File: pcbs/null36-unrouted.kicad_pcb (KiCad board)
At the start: 2 copper layers, 123.2 x 106.1 mm, 40 parts

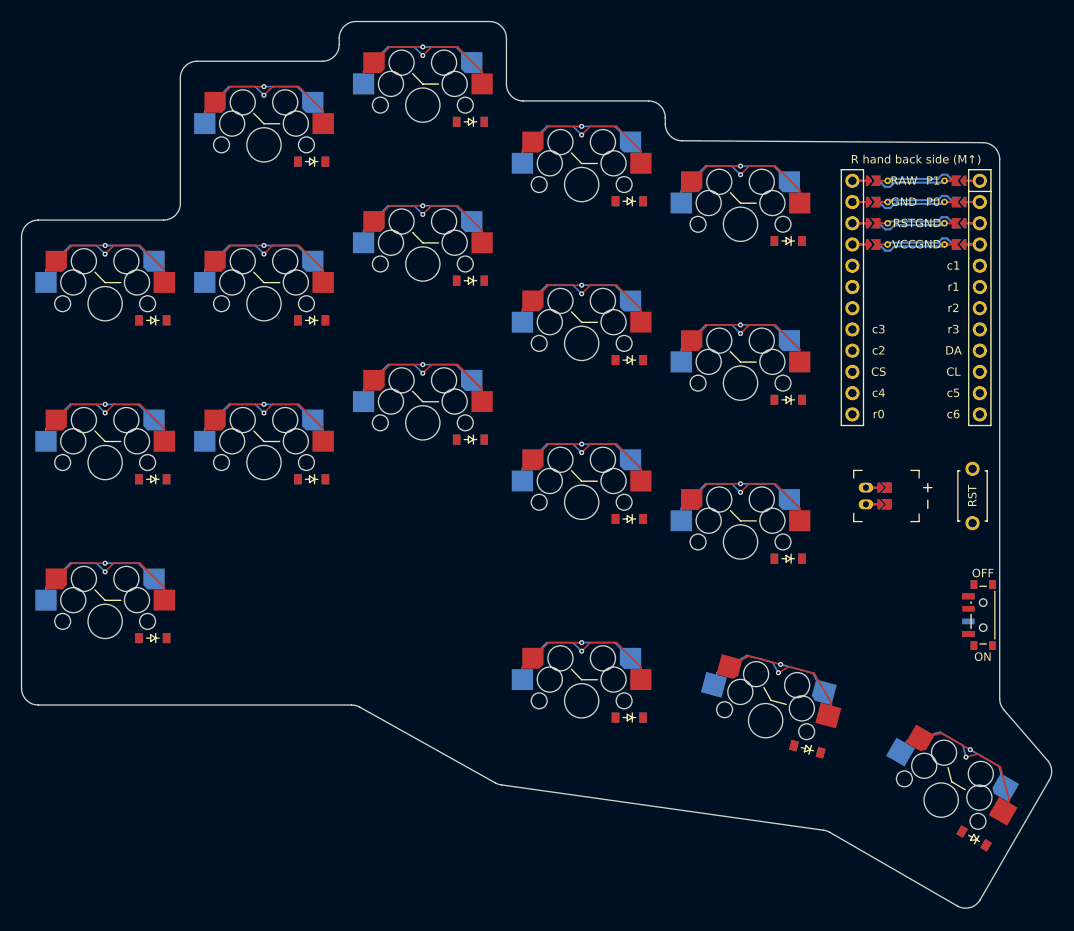
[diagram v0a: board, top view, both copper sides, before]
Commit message: v3 pcb design
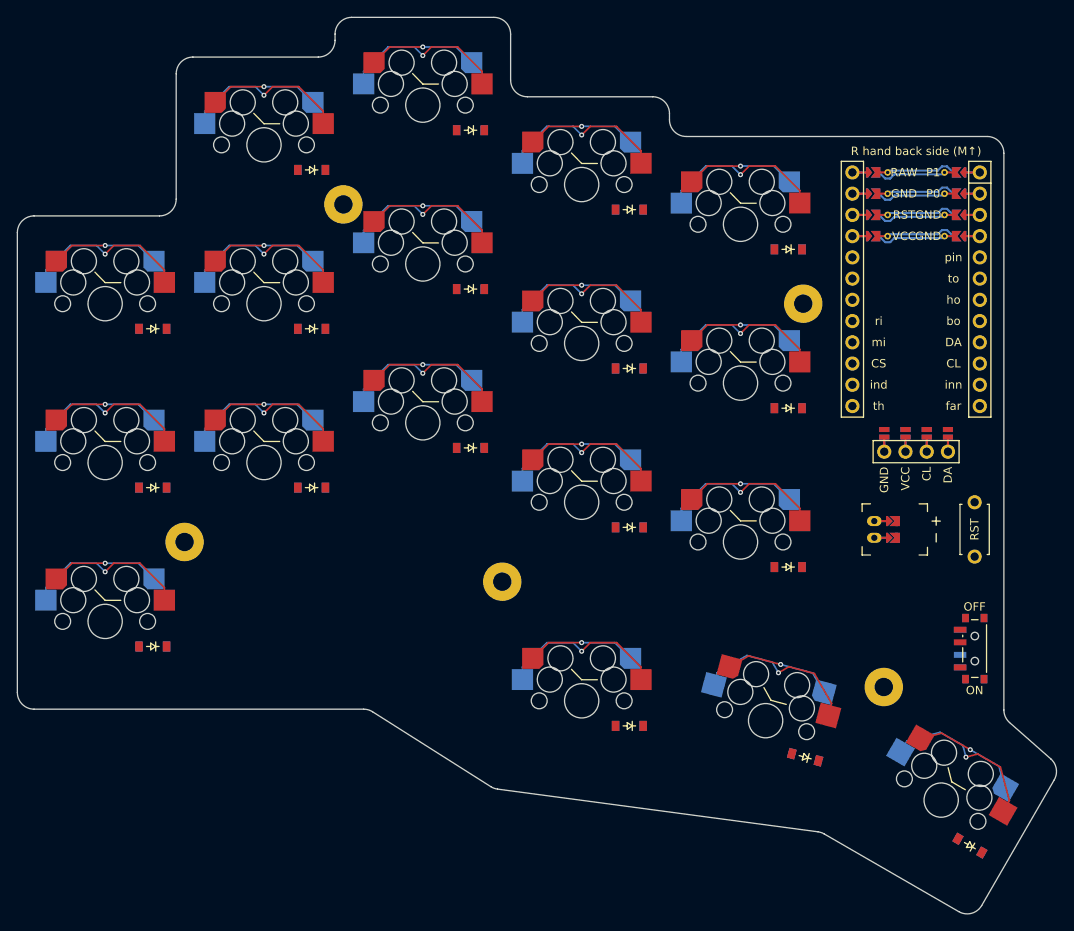
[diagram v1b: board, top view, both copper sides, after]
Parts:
- added DISP1: , ceoloide:display_ssd1306, F.Cu at (247.0, 113.0)
- added MH1: , ceoloide:mounting_hole_npth, F.Cu at (159.5, 140.5)
- added MH2: , ceoloide:mounting_hole_npth, F.Cu at (178.5, 100.1)
- added MH3: , ceoloide:mounting_hole_npth, F.Cu at (243.1, 157.8)
- added MH4: , ceoloide:mounting_hole_npth, F.Cu at (233.5, 112.0)
- added MH5: , ceoloide:mounting_hole_npth, F.Cu at (197.5, 145.2)
- moved JST1 4.12 mm to (242.0, 139.0)
- moved PWR1 4.12 mm to (254.0, 153.2)
- moved RST1 4.01 mm to (254.0, 139.0)
- moved D1 1.00 mm to (155.7, 153.0)
- moved D10 1.00 mm to (212.7, 138.8)
- moved D11 1.00 mm to (212.7, 119.8)
- moved D12 1.00 mm to (212.7, 100.8)
- moved D13 1.00 mm to (231.7, 143.5)
- moved D14 1.00 mm to (231.7, 124.5)
- moved D15 1.00 mm to (231.7, 105.5)
- moved D16 1.00 mm to (212.7, 162.5)
- moved D2 1.00 mm to (155.7, 134.0)
- moved D3 1.00 mm to (155.7, 115.0)
- moved D4 1.00 mm to (174.7, 134.0)
- moved D5 1.00 mm to (174.7, 115.0)
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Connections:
- net far_thumb renamed far_th
- net home_thumb renamed inn_th
- net index_bottom renamed ind_bo
- net index_home renamed ind_ho
- net index_top renamed ind_to
- net inner_bottom renamed inn_bo
- net inner_home renamed inn_ho
- net inner_top renamed inn_to
- net middle_bottom renamed mi_bo
- net middle_home renamed mi_ho
- net middle_top renamed mi_to
- net near_thumb renamed ind_th
- net pinky_bottom renamed pin_bo
- net pinky_home renamed pin_ho
- net pinky_top renamed pin_to
- net ring_bottom renamed ri_bo
- net ring_home renamed ri_ho
- net ring_top renamed ri_to
- D1 pad 1: bottom -> bo
- D10 pad 1: bottom -> bo
- D11 pad 1: home -> ho
- D12 pad 1: top -> to
- D13 pad 1: bottom -> bo
- D14 pad 1: home -> ho
- D15 pad 1: top -> to
- D16 pad 1: thumb -> th
- D17 pad 1: thumb -> th
- D18 pad 1: thumb -> th
- D2 pad 1: home -> ho
- D3 pad 1: top -> to
- D4 pad 1: bottom -> bo
- D5 pad 1: home -> ho
- D6 pad 1: top -> to
- D7 pad 1: bottom -> bo
- D8 pad 1: home -> ho
- D9 pad 1: top -> to
- MCU1 pad 11: c5 -> inn
- MCU1 pad 12: c6 -> far
- MCU1 pad 13: r0 -> th
- MCU1 pad 14: c4 -> ind
- MCU1 pad 16: c2 -> mi
- MCU1 pad 17: c3 -> ri
- MCU1 pad 5: c1 -> pin
- MCU1 pad 6: r1 -> to
- MCU1 pad 7: r2 -> ho
- MCU1 pad 8: r3 -> bo
- S1 pad 2: bottom -> pin
- S10 pad 2: bottom -> ind
- S11 pad 2: home -> ind
- S12 pad 2: top -> ind
- S13 pad 2: bottom -> inn
- S14 pad 2: home -> inn
- S15 pad 2: top -> inn
- S16 pad 2: thumb -> ind
- S17 pad 2: thumb -> inn
- S18 pad 2: thumb -> far
- S2 pad 2: home -> pin
- S3 pad 2: top -> pin
- S4 pad 2: bottom -> ri
- S5 pad 2: home -> ri
- S6 pad 2: top -> ri
- S7 pad 2: bottom -> mi
- S8 pad 2: home -> mi
- S9 pad 2: top -> mi
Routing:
- net bottom: track 115.5 -> 0.00 mm, vias 5 -> 0
- net home: track 115.5 -> 0.00 mm, vias 5 -> 0
- net top: track 115.5 -> 0.00 mm, vias 5 -> 0
- net inn: track 0.00 -> 92.4 mm, vias 0 -> 4
- net ind: track 0.00 -> 92.4 mm, vias 0 -> 4
- net thumb: track 69.3 -> 0.00 mm, vias 3 -> 0
- net pin: track 0.00 -> 69.3 mm, vias 0 -> 3
- net ri: track 0.00 -> 69.3 mm, vias 0 -> 3
- net mi: track 0.00 -> 69.3 mm, vias 0 -> 3
- net far: track 0.00 -> 23.1 mm, vias 0 -> 1
- net DISP1_4: track 0.00 -> 3.50 mm
- net DISP1_3: track 0.00 -> 3.50 mm
- net DISP1_2: track 0.00 -> 3.50 mm
- net DISP1_1: track 0.00 -> 3.50 mm
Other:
- board size 123.2 x 106.1 mm -> 124.3 x 107.2 mm
